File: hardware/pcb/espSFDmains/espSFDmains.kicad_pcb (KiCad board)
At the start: 2 copper layers, 69 x 65 mm, 14 parts, among them J1 Conn_01x06_Socket, J2 Conn_02x10_Odd_Even, J3 Conn_01x02_Socket, Q1 IRLU3110Z, U1 WeMos_D1_mini_esp32, U2 TSR_1-2415

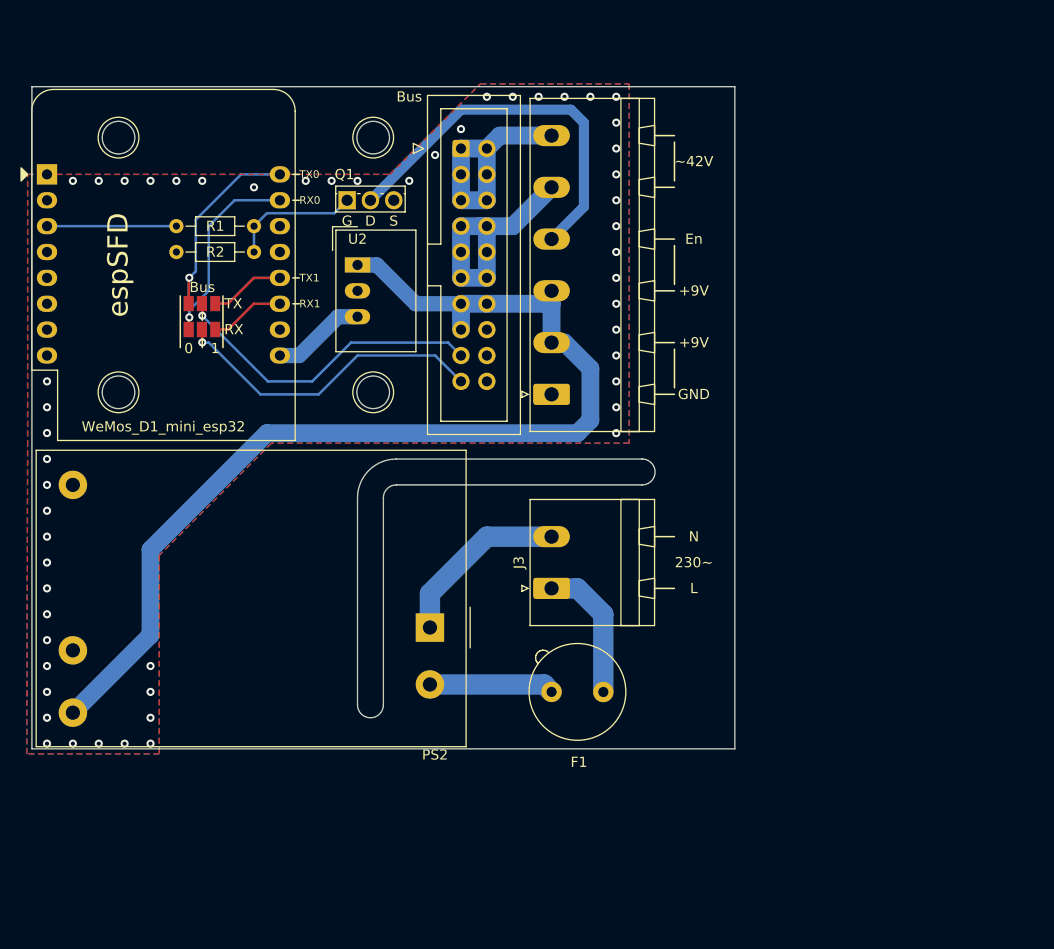
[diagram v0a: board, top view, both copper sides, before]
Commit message: ghjfgj
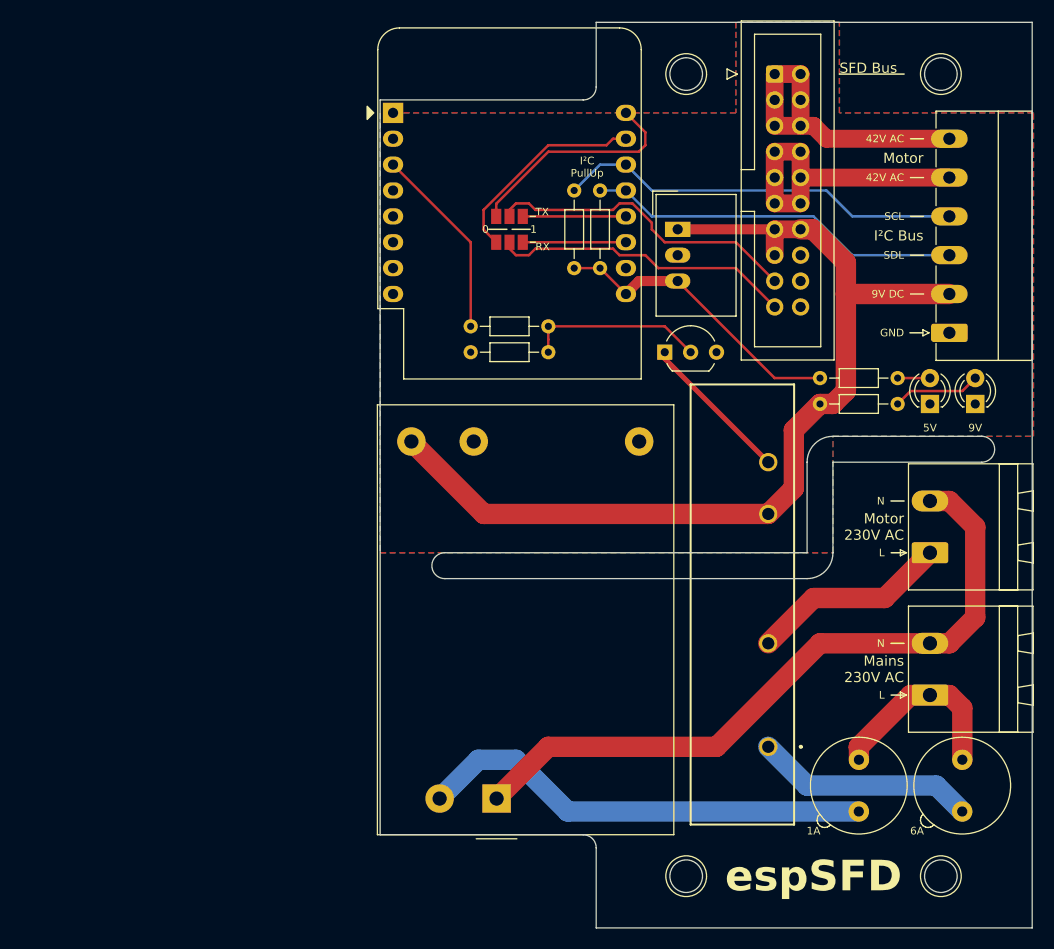
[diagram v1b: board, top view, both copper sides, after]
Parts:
- removed Q1: IRLU3110Z, PCM_Package_TO_SOT_THT_AKL:TO-251-3_Vertical_GDS
- added 5V1: LED, LED_THT:LED_D3.0mm, F.Cu at (137.5, 107.6)
- added 9V1: LED, LED_THT:LED_D3.0mm, F.Cu at (141.9, 107.6)
- added F2: 6A, Fuse:Fuseholder_TR5_Littelfuse_No560_No460, F.Cu at (140.7, 142.6)
- added J4: Mains Motor, Connector_Phoenix_MSTB:PhoenixContact_MSTBA_2,5_2-G-5,08_1x02_P5.08mm_Horizontal, F.Cu at (137.5, 122.2)
- added K1: SKB10420, KiCad:SKB10420, F.Cu at (121.6, 141.3)
- added Q2: BS170, PCM_Package_TO_SOT_THT_AKL:TO-92_Inline_Wide_DGS, F.Cu at (111.4, 102.5)
- added R3: 180R, Resistor_THT:R_Axial_DIN0204_L3.6mm_D1.6mm_P7.62mm_Horizontal, F.Cu at (134.3, 107.6)
- added R4: 180R, Resistor_THT:R_Axial_DIN0204_L3.6mm_D1.6mm_P7.62mm_Horizontal, F.Cu at (134.3, 105.1)
- added R5: 4K7, Resistor_THT:R_Axial_DIN0204_L3.6mm_D1.6mm_P7.62mm_Horizontal, F.Cu at (102.5, 86.7)
- added R6: 4K7, Resistor_THT:R_Axial_DIN0204_L3.6mm_D1.6mm_P7.62mm_Horizontal, F.Cu at (105.1, 86.7)
- J1: footprint Connector_Phoenix_MSTB:PhoenixContact_MSTBA_2,5_6-G-5,08_1x06_P5.08mm_Horizontal -> Connector_Phoenix_MC:PhoenixContact_MC_1,5_6-G-3.81_1x06_P3.81mm_Horizontal
- J3: value Conn_01x02_Socket -> Mains
- R2: value 2K2 -> 180K
- U2: value TSR_1-2415 -> TSR_1-2450
- moved DRA2 91.4 mm to (126.0, 154.0), turned to 0 degrees
- moved DRA1 63.9 mm to (126.0, 75.2), turned to 0 degrees
- moved J1 39.5 mm to (139.4, 100.6)
- moved J3 38.6 mm to (137.5, 136.2)
- moved U1 34.5 mm to (84.8, 79.0)
- moved J2 31.7 mm to (122.2, 75.2)
- moved U2 31.6 mm to (112.7, 90.5)
- moved JP2 31.4 mm to (96.2, 89.2)
- moved JP1 31.4 mm to (96.2, 91.8)
- moved R2 30.5 mm to (100.0, 102.5)
- moved R1 30.5 mm to (92.4, 100.0)
- moved F1 26.0 mm to (130.5, 142.6), turned to -90 degrees
- moved PS2 18.0 mm to (94.9, 146.4), turned to 90 degrees
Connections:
- J1 pad 3: +9V -> SDA
- J1 pad 4: En Motor -> SCL
- U1 pad 13: unconnected-(U1-SDA/D2-Pad13) -> SDA
- U1 pad 14: unconnected-(U1-SCL/D1-Pad14) -> SCL
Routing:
- net NEUT: track 17.6 -> 68.7 mm
- net SCL: track 0.00 -> 40.0 mm
- net En Motor: track 37.9 -> 0.00 mm
- net SDA: track 0.00 -> 36.9 mm
- net Net-(PS2-AC/L): track 12.2 -> 44.8 mm
- net Net-(K1-~_1): track 0.00 -> 21.7 mm
- net +5V: track 9.20 -> 29.7 mm
- net 230V Motor: track 0.00 -> 19.6 mm
- net Net-(K1--): track 0.00 -> 15.6 mm
- net Net-(9V1-A): track 0.00 -> 8.67 mm
- net +9V: track 105.8 -> 97.1 mm
- net Motor N: track 22.1 -> 30.4 mm
- net Net-(U1-D0): track 12.7 -> 19.0 mm
- net Motor L: track 23.8 -> 29.8 mm
- net LINE: track 13.8 -> 19.1 mm
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- added copper zone on F.Cu, net Motor L
- added copper zone on F.Cu, net Motor N
- removed copper zone on B.Cu, net Motor L
- removed copper zone on B.Cu, net Motor N
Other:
- board size 69 x 65 mm -> 64 x 88.9 mm
- board text added: "1A"
- board text added: "42V AC"
- board text added: "5V"
- board text added: "6A"
- board text added: "9V"
- board text added: "9V DC"
- board text added: "I²C Bus"
- board text added: "I²C PullUp"
- board text added: "Mains 230V AC"
- board text added: "Motor"
- board text added: "Motor 230V AC"
- board text added: "SCL"
- board text added: "SDL"
- board text added: "SFD Bus"
- board text removed: "+9V"
- board text removed: "230~"
- board text removed: "Bus"
- board text removed: "En"
- board text removed: "RX0"
- board text removed: "RX1"
- board text removed: "TX0"
- board text removed: "TX1"
- board text removed: "~42V"
